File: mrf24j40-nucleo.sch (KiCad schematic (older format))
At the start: 2 parts, among them M1 MRF24J40MA_TRANSEIVER_MODULE, P1 CONN_02X08

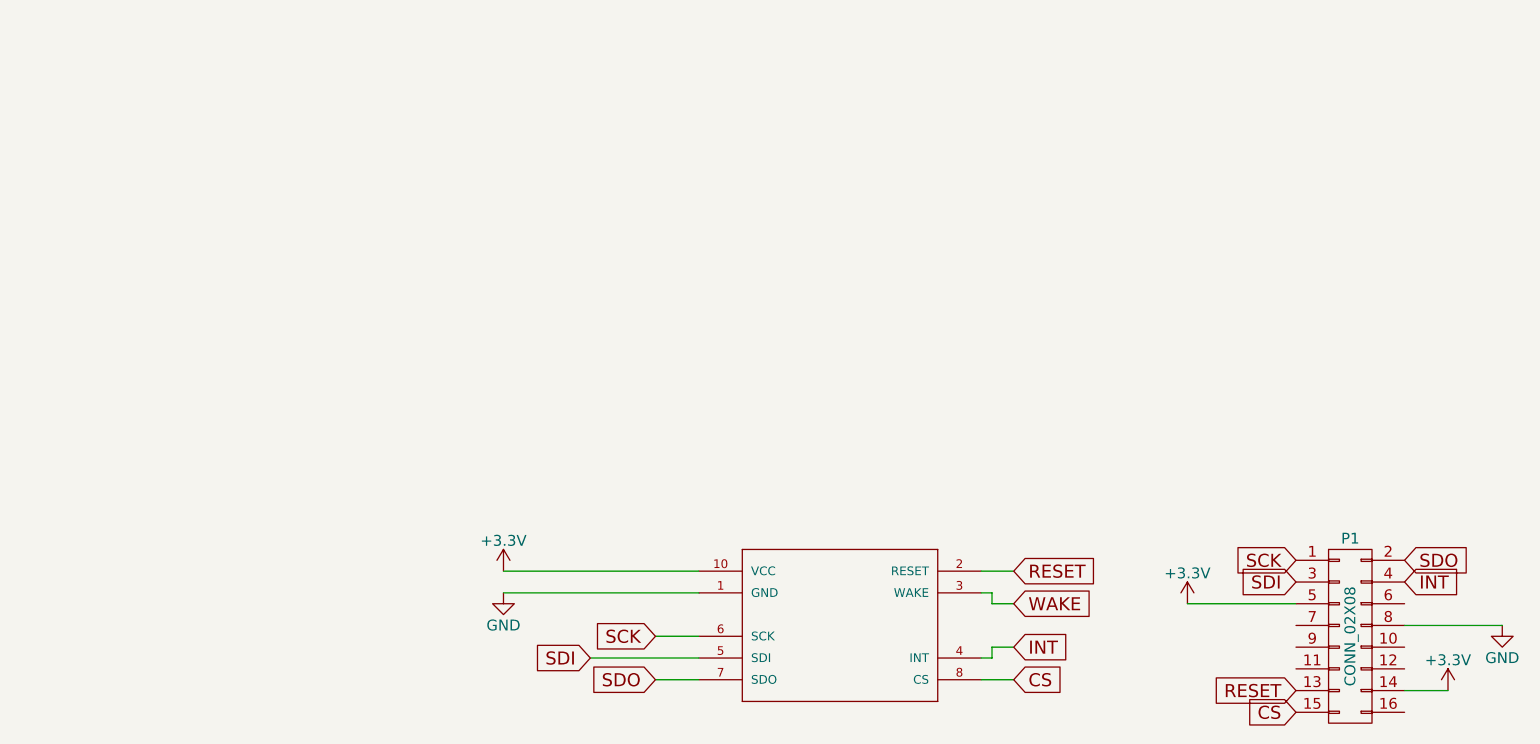
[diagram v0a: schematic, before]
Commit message: Change sheet size
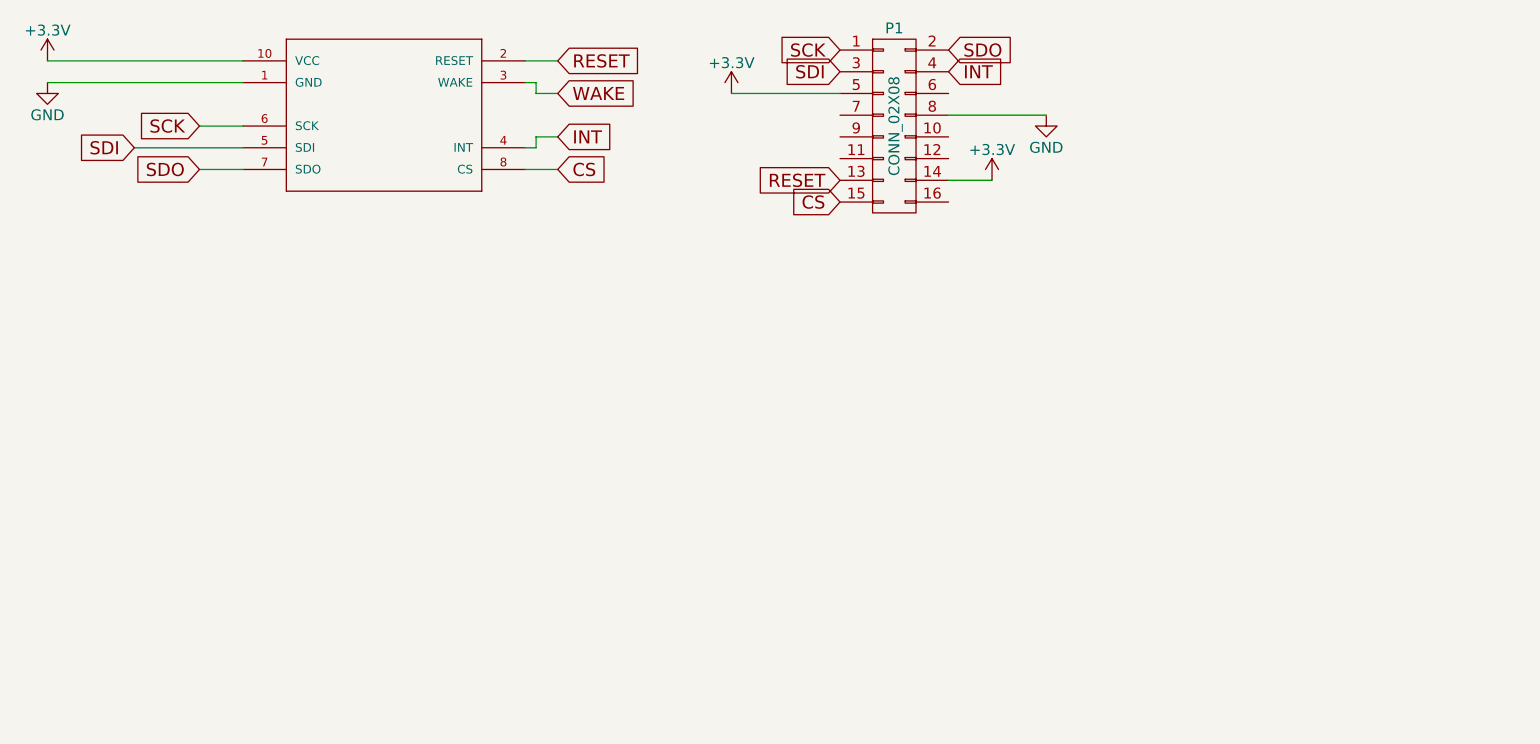
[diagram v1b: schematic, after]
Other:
- moved on the sheet: P1
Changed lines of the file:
@@
 EELAYER 25 0
 EELAYER END
-$Descr A4 11693 8268
+$Descr User 7874 4000
 encoding utf-8
 Sheet 1 1
@@
 L MRF24J40MA_TRANSEIVER_MODULE M1
 U 1 1 5884B5E6
-P 4950 3850
-F 0 "M1" H 4950 3850 45  0001 C CNN
-F 1 "MRF24J40MA_TRANSEIVER_MODULE" H 4950 3850 45  0001 C CNN
-F 2 "MRF24J40MA:MRF24J40MA-TRANSCEIVER_MODULE" H 4950 3850 60  0001 C CNN
-F 3 "" H 4950 3850 60  0000 C CNN
-	1    4950 3850
+P 2850 1500
+F 0 "M1" H 2850 1500 45  0001 C CNN
+F 1 "MRF24J40MA_TRANSEIVER_MODULE" H 2850 1500 45  0001 C CNN
+F 2 "MRF24J40MA:MRF24J40MA-TRANSCEIVER_MODULE" H 2850 1500 60  0001 C CNN
+F 3 "" H 2850 1500 60  0000 C CNN
+	1    2850 1500
 	1    0    0    -1
 $EndComp
@@
 L +3.3V #PWR01
 U 1 1 5884B64A
-P 3450 3350
-F 0 "#PWR01" H 3450 3200 50  0001 C CNN
-F 1 "+3.3V" H 3450 3490 50  0000 C CNN
-F 2 "" H 3450 3350 60  0000 C CNN
-F 3 "" H 3450 3350 60  0000 C CNN
-	1    3450 3350
+P 1350 1000
+F 0 "#PWR01" H 1350 850 50  0001 C CNN
+F 1 "+3.3V" H 1350 1140 50  0000 C CNN
+F 2 "" H 1350 1000 60  0000 C CNN
+F 3 "" H 1350 1000 60  0000 C CNN
+	1    1350 1000
 	1    0    0    -1
 $EndComp
@@
 L GND #PWR02
 U 1 1 5884B65E
-P 3450 3450
-F 0 "#PWR02" H 3450 3200 50  0001 C CNN
-F 1 "GND" H 3450 3300 50  0000 C CNN
-F 2 "" H 3450 3450 60  0000 C CNN
-F 3 "" H 3450 3450 60  0000 C CNN
-	1    3450 3450
+P 1350 1100
+F 0 "#PWR02" H 1350 850 50  0001 C CNN
+F 1 "GND" H 1350 950 50  0000 C CNN
+F 2 "" H 1350 1100 60  0000 C CNN
+F 3 "" H 1350 1100 60  0000 C CNN
+	1    1350 1100
 	1    0    0    -1
 $EndComp
-Text GLabel 4150 3650 0    60   Input ~ 0
+Text GLabel 2050 1300 0    60   Input ~ 0
 SCK
-Text GLabel 3850 3750 0    60   Input ~ 0
+Text GLabel 1750 1400 0    60   Input ~ 0
 SDI
-Text GLabel 4150 3850 0    60   Input ~ 0
+Text GLabel 2050 1500 0    60   Input ~ 0
 SDO
-Text GLabel 5800 3350 2    60   Input ~ 0
+Text GLabel 3700 1000 2    60   Input ~ 0
 RESET
-Text GLabel 5800 3700 2    60   Input ~ 0
+Text GLabel 3700 1350 2    60   Input ~ 0
 INT
-Text GLabel 5800 3500 2    60   Input ~ 0
+Text GLabel 3700 1150 2    60   Input ~ 0
 WAKE
-Text GLabel 5800 3850 2    60   Input ~ 0
+Text GLabel 3700 1500 2    60   Input ~ 0
 CS
-Text GLabel 7100 3300 0    60   Input ~ 0
+Text GLabel 5000 950  0    60   Input ~ 0
 SCK
-Text GLabel 7100 3400 0    60   Input ~ 0
+Text GLabel 5000 1050 0    60   Input ~ 0
 SDI
-Text GLabel 7600 3300 2    60   Input ~ 0
+Text GLabel 5500 950  2    60   Input ~ 0
 SDO
 $Comp
 L +3.3V #PWR03
 U 1 1 5884B9F5
-P 6600 3500
-F 0 "#PWR03" H 6600 3350 50  0001 C CNN
-F 1 "+3.3V" H 6600 3640 50  0000 C CNN
-F 2 "" H 6600 3500 60  0000 C CNN
-F 3 "" H 6600 3500 60  0000 C CNN
-	1    6600 3500
+P 4500 1150
+F 0 "#PWR03" H 4500 1000 50  0001 C CNN
+F 1 "+3.3V" H 4500 1290 50  0000 C CNN
+F 2 "" H 4500 1150 60  0000 C CNN
+F 3 "" H 4500 1150 60  0000 C CNN
+	1    4500 1150
 	1    0    0    -1
 $EndComp
@@
 L GND #PWR04
 U 1 1 5884BA92
-P 8050 3600
-F 0 "#PWR04" H 8050 3350 50  0001 C CNN
-F 1 "GND" H 8050 3450 50  0000 C CNN
-F 2 "" H 8050 3600 60  0000 C CNN
-F 3 "" H 8050 3600 60  0000 C CNN
-	1    8050 3600
+P 5950 1250
+F 0 "#PWR04" H 5950 1000 50  0001 C CNN
+F 1 "GND" H 5950 1100 50  0000 C CNN
+F 2 "" H 5950 1250 60  0000 C CNN
+F 3 "" H 5950 1250 60  0000 C CNN
+	1    5950 1250
 	1    0    0    -1
 $EndComp
 Wire Wire Line
-	4350 3350 3450 3350
+	2250 1000 1350 1000
 Wire Wire Line
-	4350 3450 3450 3450
+	2250 1100 1350 1100
 Wire Wire Line
-	4350 3650 4150 3650
+	2250 1300 2050 1300
 Wire Wire Line
-	4350 3750 3850 3750
+	2250 1400 1750 1400
 Wire Wire Line
-	4350 3850 4150 3850
+	2250 1500 2050 1500
 Wire Wire Line
-	5650 3350 5800 3350
+	3550 1000 3700 1000
 Wire Wire Line
-	5650 3450 5700 3450
+	3550 1100 3600 1100
 Wire Wire Line
-	5700 3450 5700 3500
+	3600 1100 3600 1150
 Wire Wire Line
-	5700 3500 5800 3500
+	3600 1150 3700 1150
 Wire Wire Line
-	5700 3750 5650 3750
+	3600 1400 3550 1400
 Wire Wire Line
-	5700 3750 5700 3700
+	3600 1400 3600 1350
 Wire Wire Line
-	5700 3700 5800 3700
+	3600 1350 3700 1350
 Wire Wire Line
-	5650 3850 5800 3850
+	3550 1500 3700 1500
 Wire Wire Line
-	6600 3500 7100 3500
+	4500 1150 5000 1150
 Wire Wire Line
-	7600 3600 8050 3600
+	5500 1250 5950 1250
 $Comp
 L +3.3V #PWR05
 U 1 1 5884BC0A
-P 7800 3900
-F 0 "#PWR05" H 7800 3750 50  0001 C CNN
-F 1 "+3.3V" H 7800 4040 50  0000 C CNN
-F 2 "" H 7800 3900 60  0000 C CNN
-F 3 "" H 7800 3900 60  0000 C CNN
-	1    7800 3900
+P 5700 1550
+F 0 "#PWR05" H 5700 1400 50  0001 C CNN
+F 1 "+3.3V" H 5700 1690 50  0000 C CNN
+F 2 "" H 5700 1550 60  0000 C CNN
+F 3 "" H 5700 1550 60  0000 C CNN
+	1    5700 1550
 	1    0    0    -1
 $EndComp
 Wire Wire Line
-	7800 3900 7600 3900
+	5700 1550 5500 1550
 $Comp
 L CONN_02X08 P1
 U 1 1 5884EF43
-P 7350 3650
-F 0 "P1" H 7350 4100 50  0000 C CNN
-F 1 "CONN_02X08" V 7350 3650 50  0000 C CNN
-F 2 "Pin_Headers:Pin_Header_Straight_2x08_Pitch2.54mm" H 7350 2450 50  0001 C CNN
-F 3 "" H 7350 2450 50  0000 C CNN
-	1    7350 3650
+P 5250 1300
+F 0 "P1" H 5250 1750 50  0000 C CNN
+F 1 "CONN_02X08" V 5250 1300 50  0000 C CNN
+F 2 "Pin_Headers:Pin_Header_Straight_2x08_Pitch2.54mm" H 5250 100 50  0001 C CNN
+F 3 "" H 5250 100 50  0000 C CNN
+	1    5250 1300
 	1    0    0    -1
 $EndComp
-Text GLabel 7100 4000 0    60   Input ~ 0
+Text GLabel 5000 1650 0    60   Input ~ 0
 CS
-Text GLabel 7600 3400 2    60   Input ~ 0
+Text GLabel 5500 1050 2    60   Input ~ 0
 INT
-Text GLabel 7100 3900 0    60   Input ~ 0
+Text GLabel 5000 1550 0    60   Input ~ 0
 RESET
 $EndSCHEMATC
